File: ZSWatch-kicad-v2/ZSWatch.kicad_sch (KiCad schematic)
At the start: 71 parts, among them IC1 ESDALC6V1W5, IC2 XC9265C181MR-G, IC3 TPS61023DRLT, IC4 MAX30101EFD+T, IC5 FAN5622SX, IC6 BMI270, IC7 LIS2MDLTR, J2 Charger and programming heade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, M1 Vibrator DC Motor, U1 MAX1811ESA+, U10 0_NORA-B106, U11 NTS0104GU12, U13 GC9A01A_CST816S, U2 DMC2400UV-7, U3 NCV300LSN36T1G, U4 BMP581, U5 BME688, U6 DRV2603RUNT, U7 XC9265A331MR-G

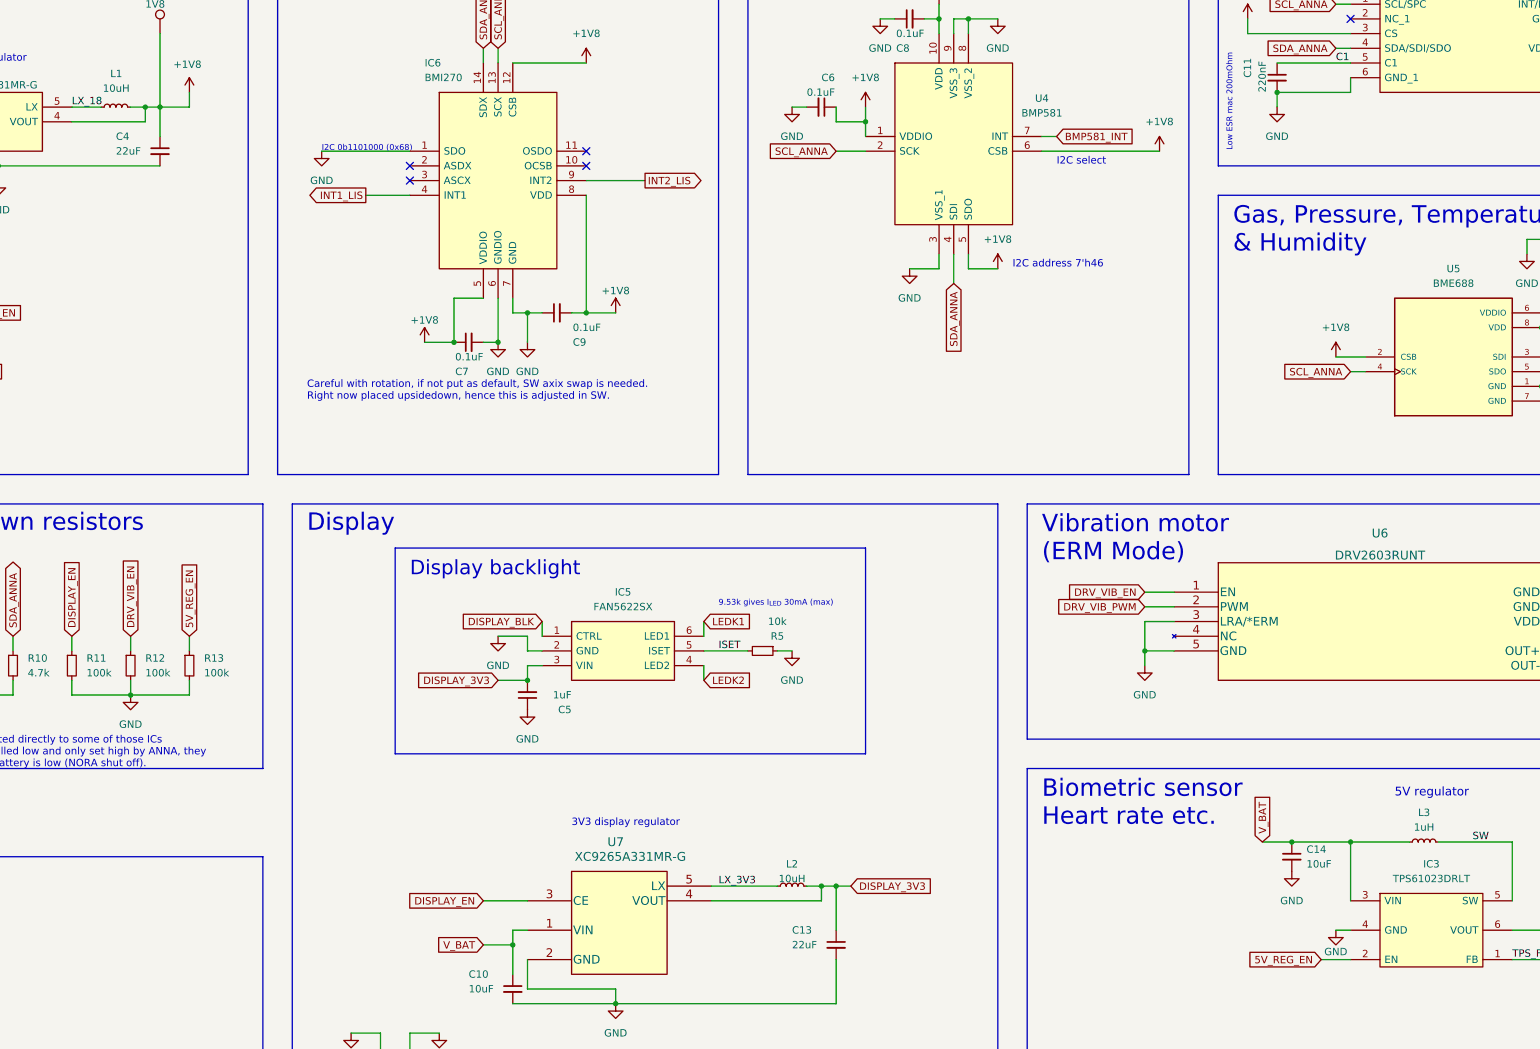
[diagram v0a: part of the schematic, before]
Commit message: test differences
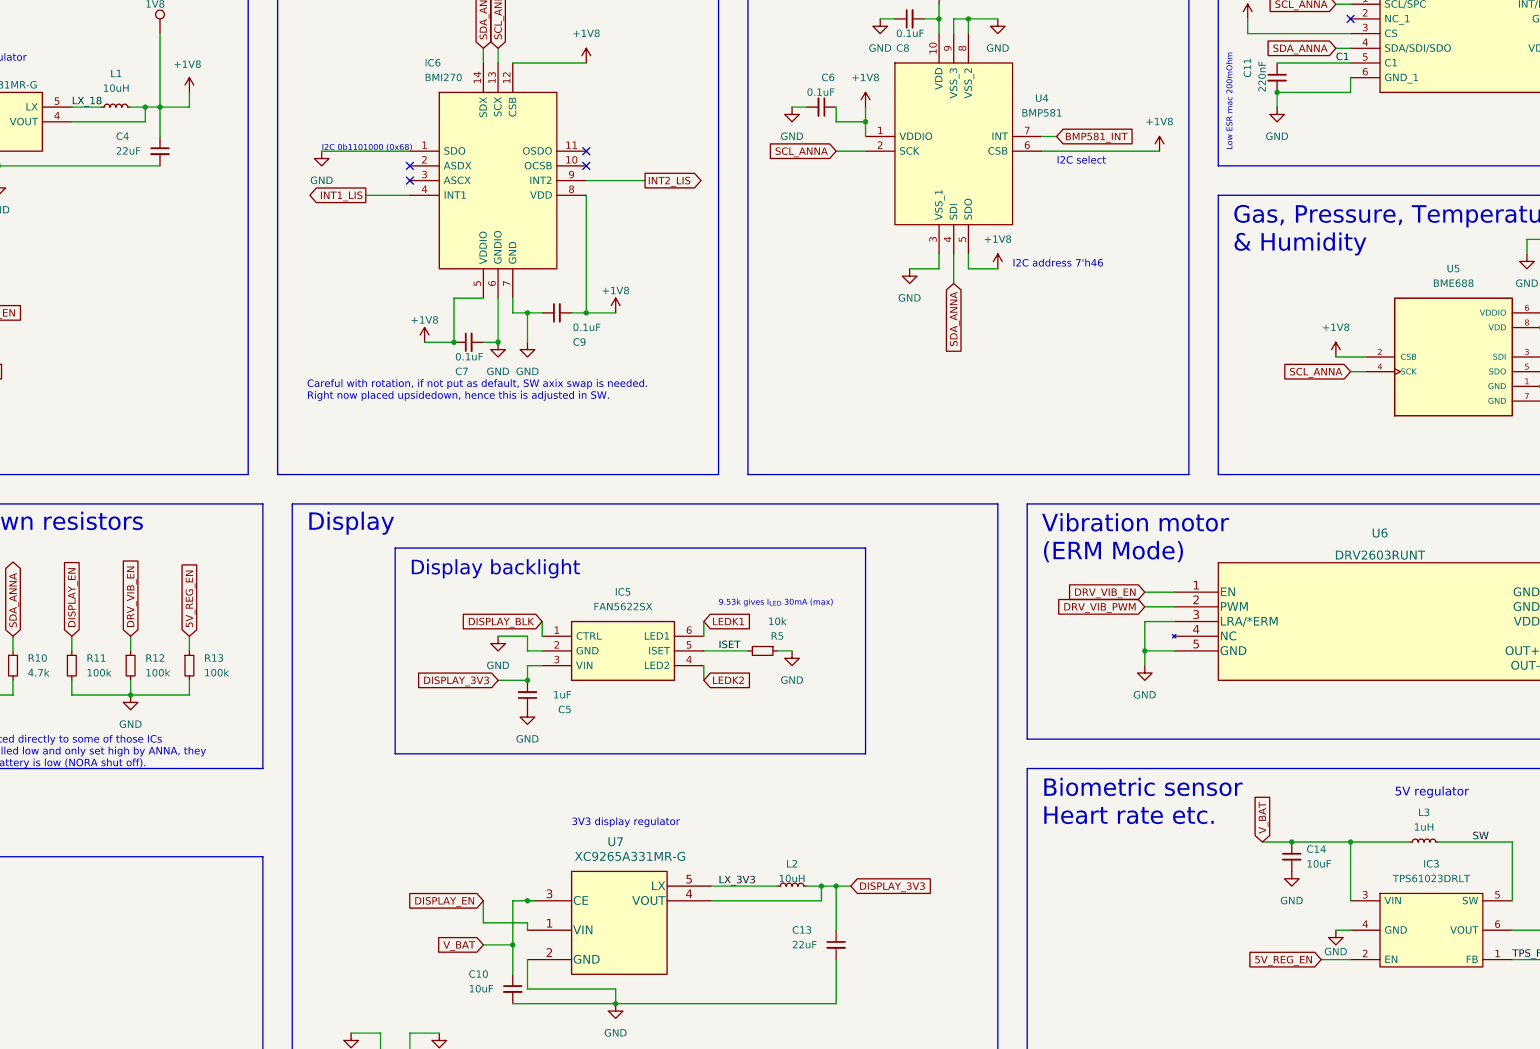
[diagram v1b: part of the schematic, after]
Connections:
- net +BATT: now also U7.3 (CE); no longer U7.1 (VIN)
- net DISPLAY_EN: now also U7.1 (VIN); no longer U7.3 (CE)
